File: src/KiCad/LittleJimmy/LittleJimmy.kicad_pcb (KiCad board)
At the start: 2 copper layers, 37.5 x 12.7 mm, 9 parts, among them J1 Conn_01x03, J2 Conn_01x04, Q1 BT169B

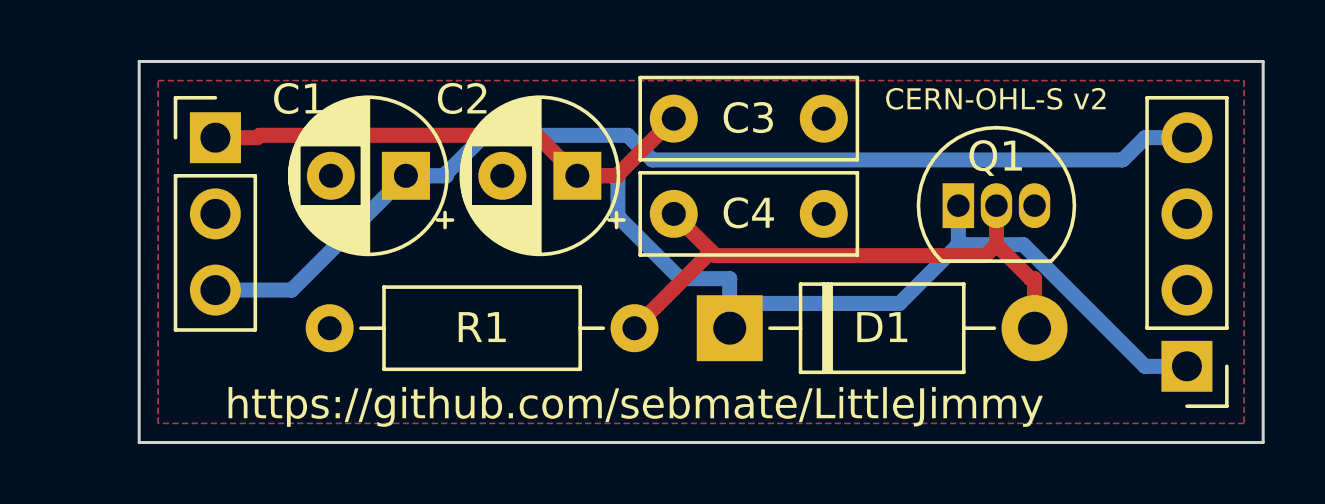
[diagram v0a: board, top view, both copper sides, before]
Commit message: Update to Version 2
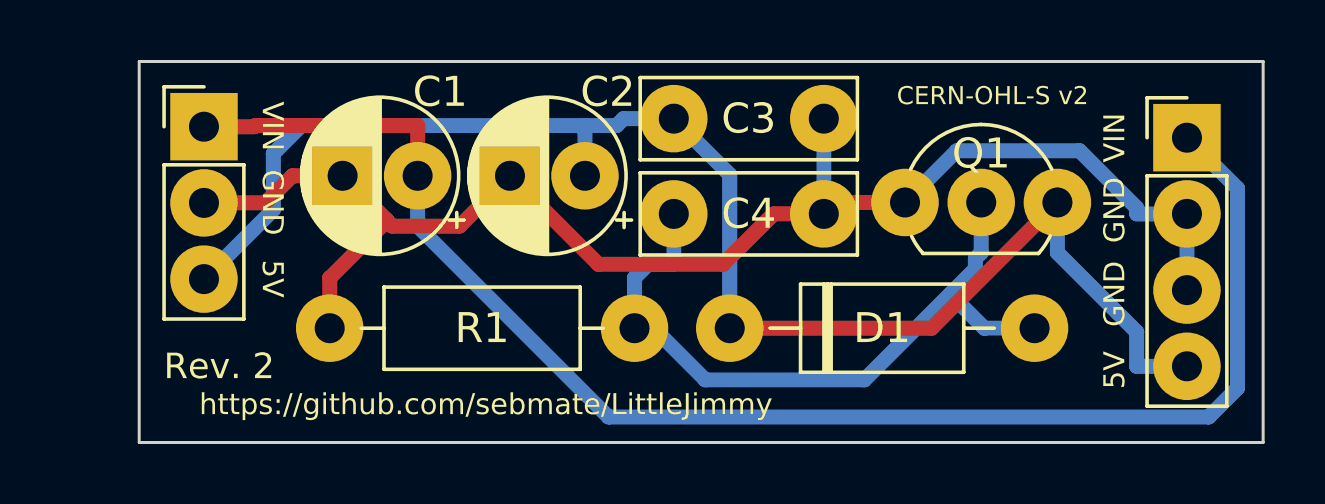
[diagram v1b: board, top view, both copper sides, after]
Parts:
- Q1: footprint Package_TO_SOT_THT:TO-92_Inline -> Package_TO_SOT_THT:TO-92L_Inline_Wide
- moved J2 7.62 mm to (83.8, 31.1), turned to 0 degrees
- moved Q1 1.78 mm to (74.4, 33.3)
- moved J1 0.53 mm to (51.1, 30.7)
- moved C1 0.39 mm to (58.2, 32.4)
- moved C2 0.25 mm to (63.8, 32.4)
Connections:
- J1 pad 1: +5V -> VCC
- J1 pad 3: VCC -> +5V
- J2 pad 1: +5V -> VCC
- J2 pad 4: VCC -> +5V
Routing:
- net GND: track 0.00 -> 48.4 mm
- net VCC: track 35.2 -> 49.9 mm
- net +5V: track 44.7 -> 49.3 mm
- net Net-(C4-Pad1): track 19.8 -> 24.3 mm
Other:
- board text added: "5V"
- board text added: "GND"
- board text added: "Rev. 2"
- board text added: "VIN"
